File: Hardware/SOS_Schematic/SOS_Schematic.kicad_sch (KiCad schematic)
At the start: 26 parts, among them J1 USB_B_Mini, J2 Conn_02x07_Odd_Even, U1 MCP1802x-xx02xOT, U2 STM32L476RGTx, U3 HTRC11001T, Y1 Crystal_Small

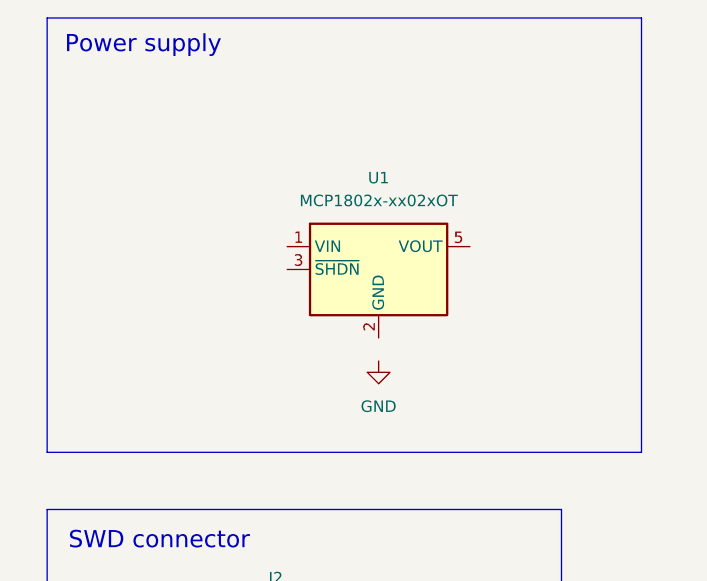
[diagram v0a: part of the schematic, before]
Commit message: power supply schematic
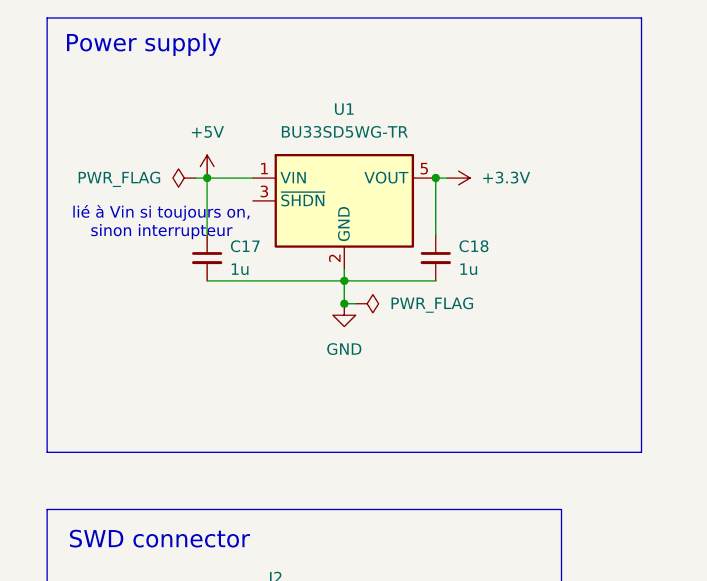
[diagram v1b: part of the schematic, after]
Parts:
- added C17, C18: 1u, symbol Device:C_Small
- U1: value MCP1802x-xx02xOT -> BU33SD5WG-TR
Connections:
- net +3.3V: now also U1.5 (VOUT), C18.1
- net GND: now also U1.2 (GND), C17.2, C18.2
- net +5V: now reaches U1.1 (VIN)
- net +5V: now also C17.1
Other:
- note added: "lié à Vin si toujours on, sinon interrupteur"
- moved on the sheet: U1
